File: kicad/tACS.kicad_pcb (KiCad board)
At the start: 2 copper layers, 26 parts, among them J1 +35V, J2 -35V, J3 GND/ELETRODO(-), J4 METER(+), J5 ENTRADA SINAL, J6 METER(-), J7 ELETRODO(+), Q1 TIP42C, Q2 TIP41C, Q3 2N5401, Q4 2N5551, U1 LM741, U2 LM741

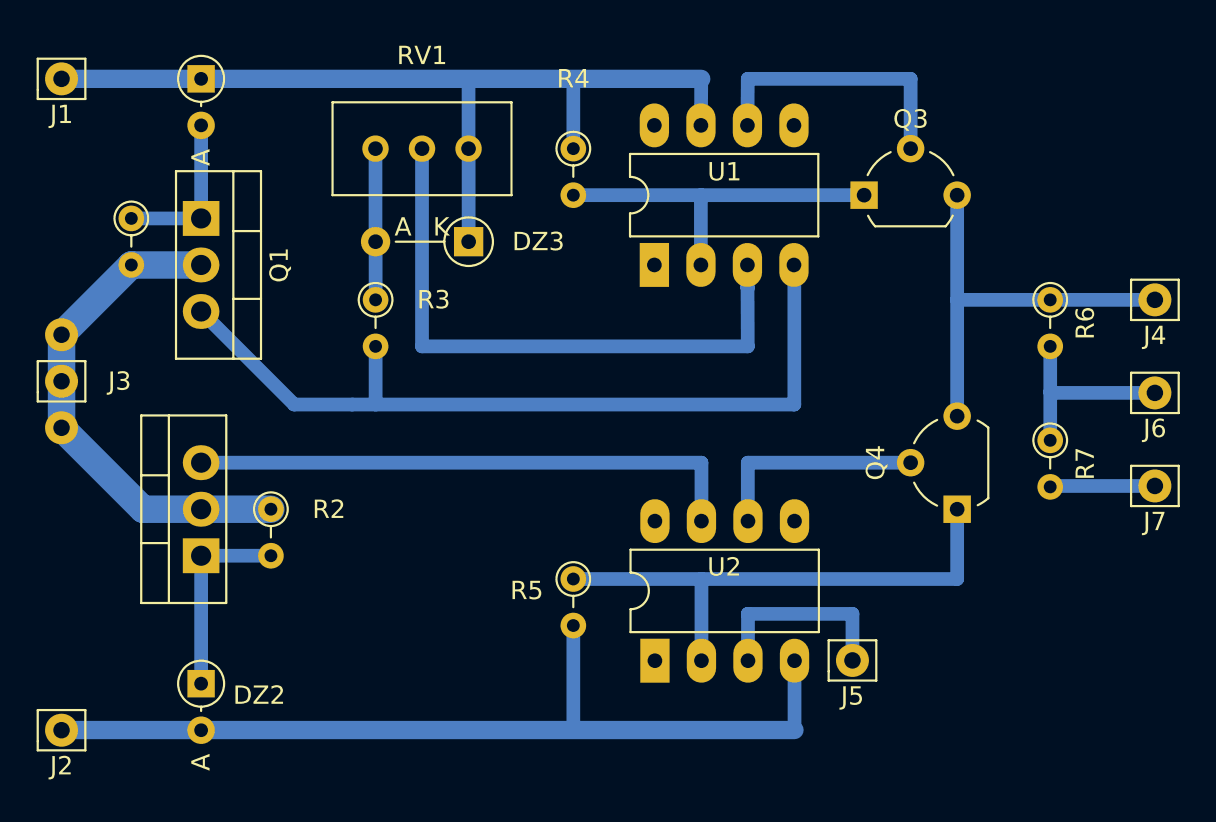
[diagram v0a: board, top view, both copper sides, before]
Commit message: Add files via upload
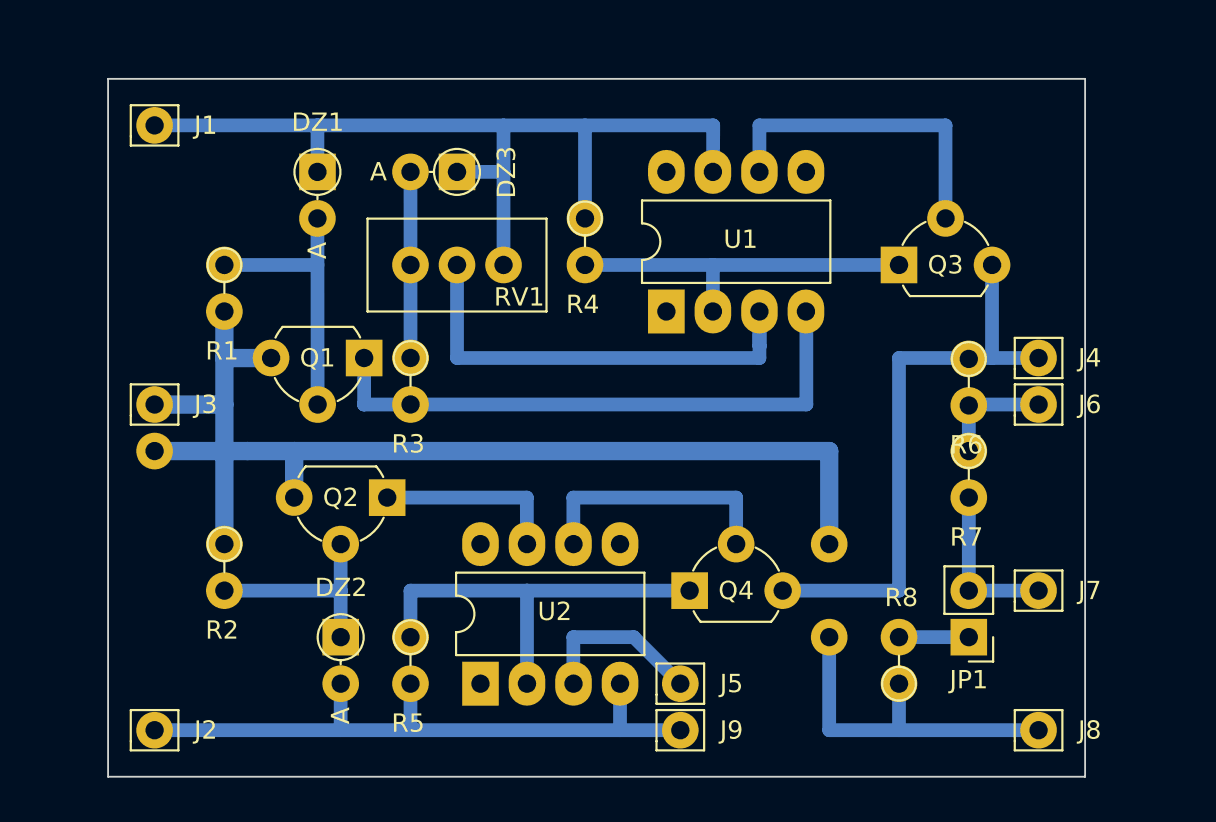
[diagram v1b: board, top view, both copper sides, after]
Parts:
- removed the ? at (119.4, 80.0)
- removed the ? at (119.4, 74.9)
- added ?: , , F.Cu at (124.5, 81.3)
- added ?: , , F.Cu at (161.3, 86.4)
- added ?: , , F.Cu at (161.3, 91.4)
- added J8: ELETRODO(-), tACS:Pin_D0.9mm_L10.0mm_W2.4mm_FlatFork, F.Cu at (172.7, 96.5)
- added J9: S-, tACS:Pin_D0.9mm_L10.0mm_W2.4mm_FlatFork, F.Cu at (153.2, 96.5)
- added JP1: teste, tACS:PinHeader_1x02_P2.54mm_Vertical, F.Cu at (168.9, 91.4)
- added R8: 10K, tACS:R_Axial_DIN0204_L3.6mm_D1.6mm_P2.54mm_Vertical, F.Cu at (165.1, 94.0)
- DZ1, DZ2: footprint Diode_THT:D_DO-34_SOD68_P2.54mm_Vertical_AnodeUp -> tACS:D_DO-34_SOD68_P2.54mm_Vertical_AnodeUp
- DZ3: footprint Diode_THT:D_DO-35_SOD27_P5.08mm_Vertical_AnodeUp -> tACS:D_DO-34_SOD68_P2.54mm_Vertical_AnodeUp
- J1, J2, J4, J6, J7: footprint Connector_Pin:Pin_D0.9mm_L10.0mm_W2.4mm_FlatFork -> tACS:Pin_D0.9mm_L10.0mm_W2.4mm_FlatFork
- J3: value GND/ELETRODO(-) -> GND; footprint Connector_Pin:Pin_D0.9mm_L10.0mm_W2.4mm_FlatFork -> tACS:Pin_D0.9mm_L10.0mm_W2.4mm_FlatFork
- J5: value ENTRADA SINAL -> S+; footprint Connector_Pin:Pin_D0.9mm_L10.0mm_W2.4mm_FlatFork -> tACS:Pin_D0.9mm_L10.0mm_W2.4mm_FlatFork
- Q1: value TIP42C -> 2N5401; footprint Package_TO_SOT_THT:TO-220-3_Vertical -> tACS:TO-92L_Wide
- Q2: value TIP41C -> 2N5551; footprint Package_TO_SOT_THT:TO-220-3_Vertical -> tACS:TO-92L_Wide
- Q3, Q4: footprint Package_TO_SOT_THT:TO-92L_Wide -> tACS:TO-92L_Wide
- R1, R2, R3, R4, R5, R6, R7: footprint Resistor_THT:R_Axial_DIN0204_L3.6mm_D1.6mm_P2.54mm_Vertical -> tACS:R_Axial_DIN0204_L3.6mm_D1.6mm_P2.54mm_Vertical
- RV1: footprint Potentiometer_THT:Potentiometer_Bourns_3296W_Vertical -> tACS:Potentiometer_Bourns_3296W_Vertical
- U1: footprint Package_DIP:DIP-8_W7.62mm_LongPads -> tACS:DIP-8_W7.62mm_LongPads
- moved Q4 15.3 mm to (153.7, 88.9), turned to 0 degrees
- moved Q1 11.7 mm to (135.9, 76.2), turned to 180 degrees
- moved Q2 10.6 mm to (137.2, 83.8), turned to 180 degrees
- moved U2 9.61 mm to (142.2, 94.0)
- moved J5 9.48 mm to (153.2, 94.0)
- moved R5 9.44 mm to (138.4, 91.4)
- moved J7 8.54 mm to (172.7, 88.9)
- moved DZ1 8.13 mm to (133.3, 66.0)
- moved DZ2 8.03 mm to (134.6, 91.4)
- moved J4 7.10 mm to (172.7, 76.2)
- moved RV1 6.63 mm to (143.5, 71.1)
- moved J6 6.38 mm to (172.7, 78.7)
- moved R1 5.68 mm to (128.3, 71.1)
- moved J1 5.68 mm to (124.5, 63.5)
- moved R6 5.49 mm to (168.9, 76.2)
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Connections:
- Q1 pad 1: Net-(DZ1-A) -> Net-(U1-V-)
- Q1 pad 2: Net-(J3-Pin_1) -> Net-(DZ1-A)
- Q1 pad 3: Net-(Q1-E) -> Net-(J3-Pin_1)
- Q2 pad 1: Net-(DZ2-K) -> Net-(U2-V+)
- Q2 pad 2: Net-(J3-Pin_1) -> Net-(DZ2-K)
- Q2 pad 3: Net-(Q2-E) -> Net-(J3-Pin_1)
- R3 pad 2: Net-(Q1-E) -> Net-(U1-V-)
- U1 pad 4: Net-(Q1-E) -> Net-(U1-V-)
- U2 pad 7: Net-(Q2-E) -> Net-(U2-V+)
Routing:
- net Net-(J3-Pin_1): track 27.5 -> 82.6 mm
- net Net-(Q1-E): track 45.3 -> 0.00 mm
- net Net-(U1-V-): track 0.00 -> 31.2 mm
- net Net-(Q2-E): track 30.5 -> 0.00 mm
- net Net-(DZ2-A): track 49.5 -> 36.3 mm
- net Net-(U2-V+): track 0.00 -> 10.2 mm
- net Net-(U1-+): track 34.3 -> 24.8 mm
- net Net-(J4-Pin_1): track 22.9 -> 31.8 mm
- net Net-(U2--): track 29.2 -> 22.9 mm
- net Net-(DZ1-A): track 8.89 -> 15.2 mm
- net Net-(J6-Pin_1): track 10.9 -> 6.30 mm
- net Net-(JP1-A): track 0.00 -> 3.81 mm
- net Net-(J7-Pin_1): track 5.74 -> 8.89 mm
- net Net-(Q3-Pad2): track 15.2 -> 17.8 mm
- net Net-(DZ3-A): track 8.26 -> 10.2 mm
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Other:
- board outline added: 53.3 x 38.1 mm
